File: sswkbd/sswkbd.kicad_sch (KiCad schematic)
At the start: 238 parts, among them SW1 SW_PUSH, SW10 SW_PUSH, SW11 SW_PUSH, SW12 SW_PUSH, SW13 SW_PUSH, SW14 SW_PUSH, SW15 SW_PUSH, SW16 SW_PUSH, SW17 SW_PUSH, SW18 SW_PUSH, SW19 SW_PUSH, SW2 SW_PUSH, SW20 SW_PUSH, SW21 SW_PUSH, SW22 SW_PUSH, SW23 SW_PUSH, SW24 SW_PUSH, SW25 SW_PUSH, SW26 SW_PUSH, SW27 SW_PUSH, SW28 SW_PUSH, SW29 SW_PUSH, SW3 SW_PUSH, SW30 SW_PUSH, SW31 SW_PUSH, SW32 SW_PUSH, SW33 SW_PUSH, SW34 SW_PUSH, SW35 SW_PUSH, SW36 SW_PUSH, SW37 SW_PUSH, SW38 SW_PUSH, SW39 SW_PUSH, SW4 SW_PUSH, SW40 SW_PUSH, SW41 SW_PUSH, SW42 SW_PUSH, SW43 SW_PUSH, SW44 SW_PUSH, SW45 SW_PUSH, SW46 SW_PUSH, SW47 SW_PUSH, SW48 SW_PUSH, SW49 SW_PUSH, SW5 SW_PUSH, SW50 SW_PUSH, SW51 SW_PUSH, SW52 SW_PUSH, SW53 SW_PUSH, SW54 SW_PUSH, SW55 SW_PUSH, SW56 SW_PUSH, SW57 SW_PUSH, SW58 SW_PUSH, SW59 SW_PUSH, SW6 SW_PUSH, SW60 SW_PUSH, SW61 SW_PUSH, SW62 SW_PUSH, SW63 SW_PUSH, SW64 SW_PUSH, SW65 SW_PUSH, SW66 SW_PUSH, SW67 SW_PUSH, SW68 SW_PUSH, SW69 SW_PUSH, SW7 SW_PUSH, SW70 SW_PUSH, SW71 SW_PUSH, SW72 SW_PUSH, SW73 SW_PUSH, SW74 SW_PUSH, SW75 SW_PUSH, SW76 SW_PUSH, SW77 SW_PUSH, SW78 SW_PUSH, SW79 SW_PUSH, SW8 SW_PUSH, SW9 SW_PUSH, U1 ProMicro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

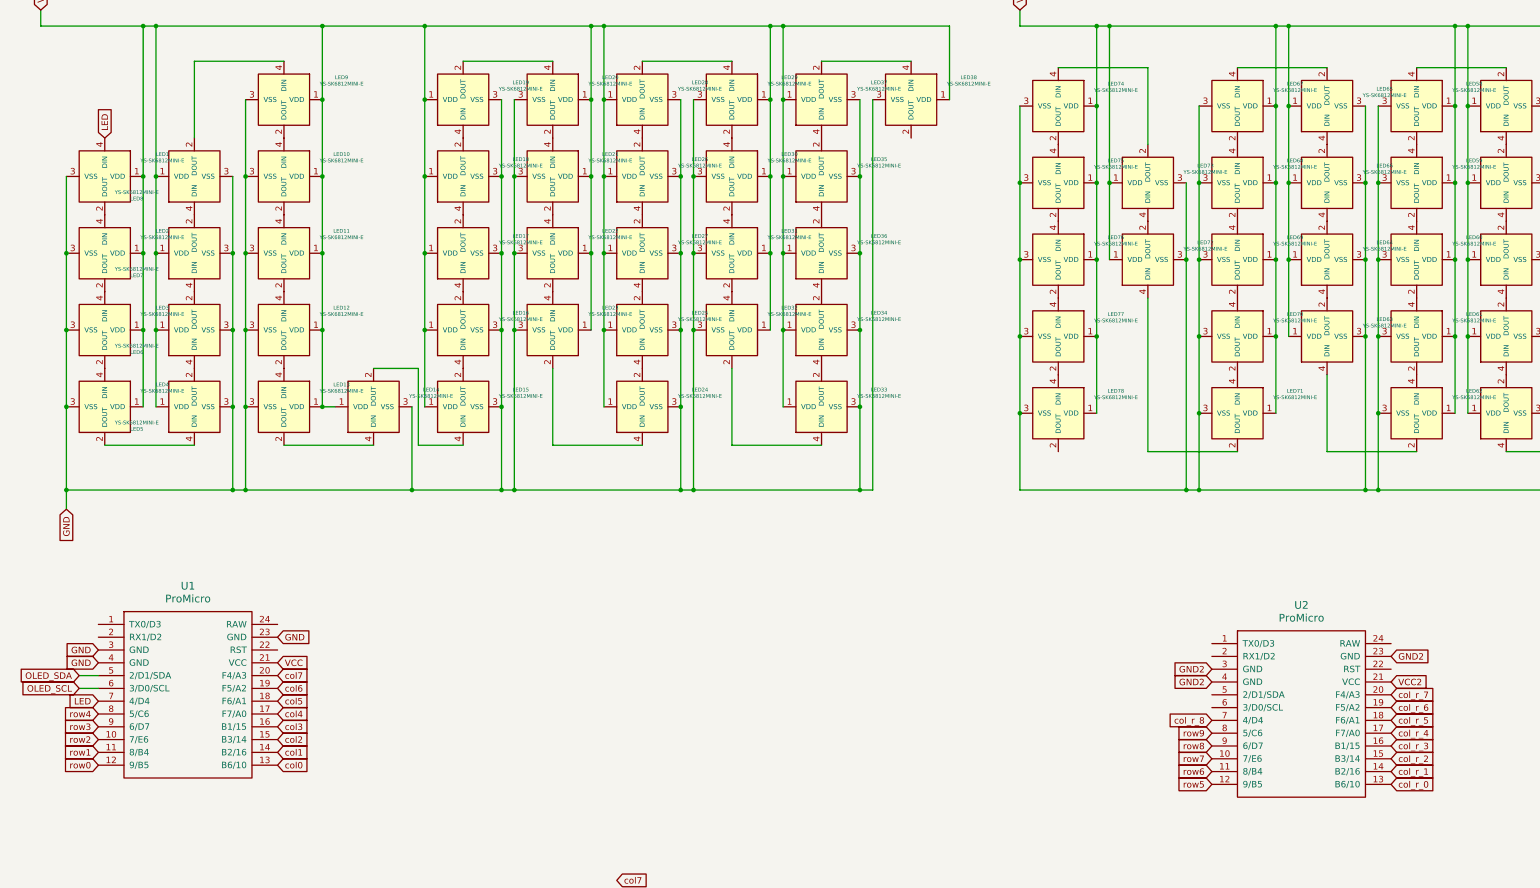
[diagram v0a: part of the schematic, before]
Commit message: wiring WIP
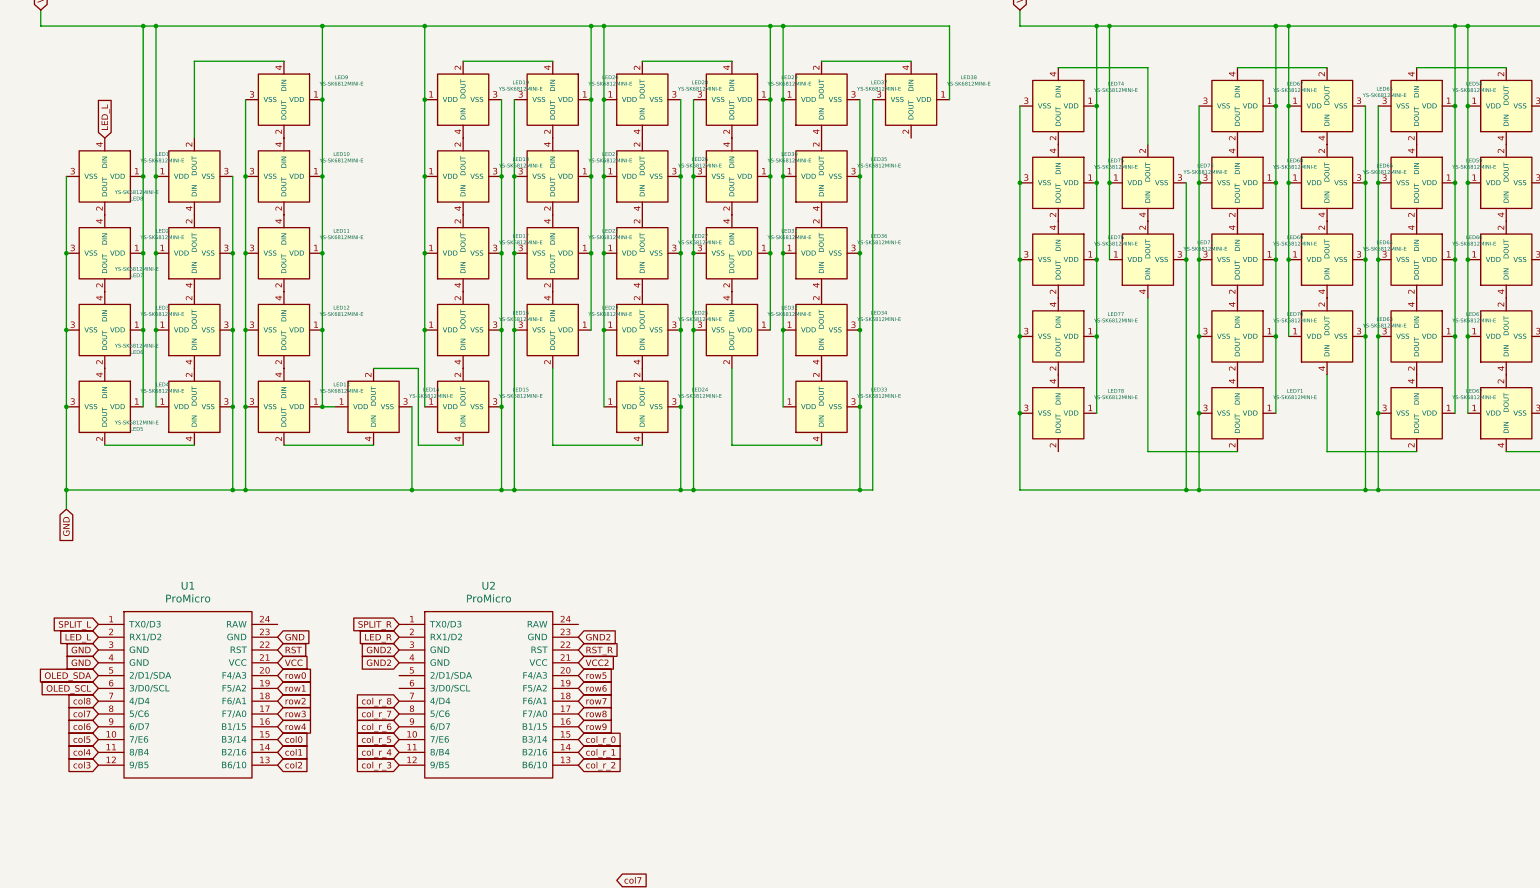
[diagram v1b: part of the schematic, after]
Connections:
- net col0: now also U1.15 (B3/14); no longer U1.13 (B6/10)
- net col2: now also U1.13 (B6/10); no longer U1.15 (B3/14)
- net col3: now also U1.12 (9/B5); no longer U1.16 (B1/15)
- net col4: now also U1.11 (8/B4); no longer U1.17 (F7/A0)
- net col5: now also U1.10 (7/E6); no longer U1.18 (F6/A1)
- net col6: now also U1.9 (6/D7); no longer U1.19 (F5/A2)
- net col7: now also U1.8 (5/C6); no longer U1.20 (F4/A3)
- net col_r_0: now also U2.15 (B3/14); no longer U2.13 (B6/10)
- net col_r_2: now also U2.13 (B6/10); no longer U2.15 (B3/14)
- net col_r_3: now also U2.12 (9/B5); no longer U2.16 (B1/15)
- net col_r_4: now also U2.11 (8/B4); no longer U2.17 (F7/A0)
- net col_r_5: now also U2.10 (7/E6); no longer U2.18 (F6/A1)
- net col_r_6: now also U2.9 (6/D7); no longer U2.19 (F5/A2)
- net col_r_7: now also U2.8 (5/C6); no longer U2.20 (F4/A3)
- net row0: now also U1.20 (F4/A3); no longer U1.12 (9/B5)
- net row1: now also U1.19 (F5/A2); no longer U1.11 (8/B4)
- net row2: now also U1.18 (F6/A1); no longer U1.10 (7/E6)
- net row3: now also U1.17 (F7/A0); no longer U1.9 (6/D7)
- net row4: now also U1.16 (B1/15); no longer U1.8 (5/C6)
- net row5: now also U2.20 (F4/A3); no longer U2.12 (9/B5)
- net row6: now also U2.19 (F5/A2); no longer U2.11 (8/B4)
- net row7: now also U2.18 (F6/A1); no longer U2.10 (7/E6)
- net row8: now also U2.17 (F7/A0); no longer U2.9 (6/D7)
- net row9: now also U2.16 (B1/15); no longer U2.8 (5/C6)
- net SPLIT_R: now reaches U2.1 (TX0/D3)
- net LED_R: now reaches U2.2 (RX1/D2)
- net RST_R: now reaches U2.22 (RST)
- net SPLIT_L: now reaches U1.1 (TX0/D3)
- net LED_L: now reaches U1.2 (RX1/D2)
- net LED_L: now also LED1.4 (DIN)
- net RST: now reaches U1.22 (RST)
- net LED renamed col8
- net col8: no longer LED1.4 (DIN)
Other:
- moved on the sheet: U2
